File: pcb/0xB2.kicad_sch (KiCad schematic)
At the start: 40 parts, among them J1 USB_C_Receptacle_USB2.0, J2 Conn_01x12, J3 Conn_01x05, J4 Conn_01x12, J5 Conn_01x02, SW1 SW_Push, SW2 SW_Push, U1 RP2040, U2 GD25Q80CEIGR, U3 XC6210B332MR-G, Y1 Crystal_GND24

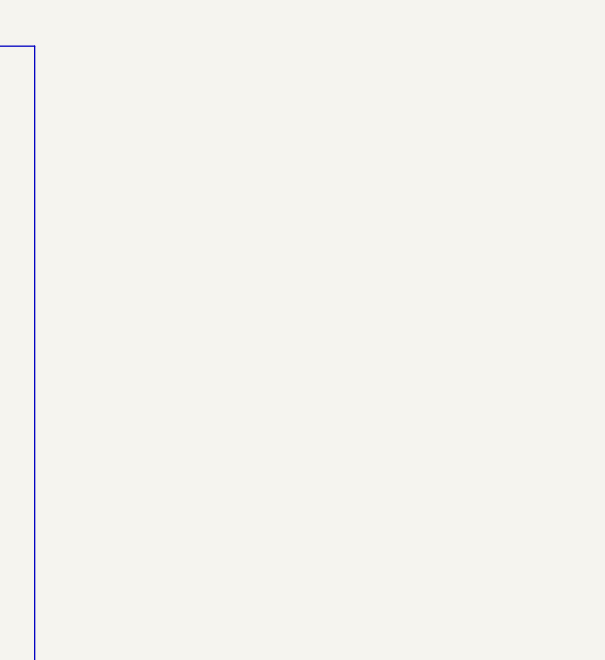
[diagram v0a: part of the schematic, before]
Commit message: import
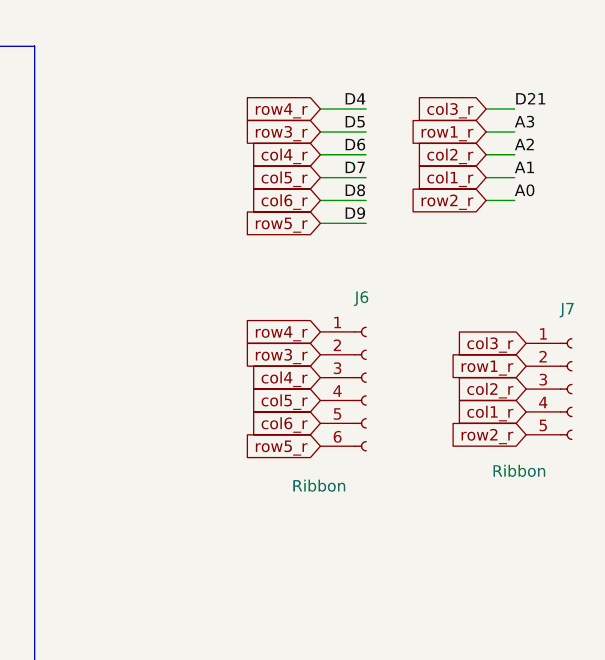
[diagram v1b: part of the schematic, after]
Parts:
- added J6: Ribbon, Connector_PinHeader_2.54mm:PinHeader_1x06_P2.54mm_Vertical, symbol Connector:Conn_01x06_Female
- added J7: Ribbon, Connector_PinHeader_2.54mm:PinHeader_1x05_P2.54mm_Vertical, symbol Connector:Conn_01x05_Female
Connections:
- net A0 renamed row2_r
- net row2_r: now also J7.5 (Pin_5)
- net A1 renamed col1_r
- net col1_r: now also J7.4 (Pin_4)
- net A2 renamed col2_r
- net col2_r: now also J7.3 (Pin_3)
- net A3 renamed row1_r
- net row1_r: now also J7.2 (Pin_2)
- net D21 renamed col3_r
- net col3_r: now also J7.1 (Pin_1)
- net D4 renamed row4_r
- net row4_r: now also J6.1 (Pin_1)
- net D5 renamed row3_r
- net row3_r: now also J6.2 (Pin_2)
- net D6 renamed col4_r
- net col4_r: now also J6.3 (Pin_3)
- net D7 renamed col5_r
- net col5_r: now also J6.4 (Pin_4)
- net D8 renamed col6_r
- net col6_r: now also J6.5 (Pin_5)
- net D9 renamed row5_r
- net row5_r: now also J6.6 (Pin_6)
